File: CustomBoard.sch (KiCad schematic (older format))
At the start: 36 parts, among them J1 RIGHT, J10 Sensor08, J11 Sensor09, J12 Sensor10, J13 Sensor11, J14 Sensor12, J15 Camera, J2 LEFT, J3 Sensor01, J4 Sensor02, J5 Sensor03, J6 Sensor04, J7 Sensor05, J8 Sensor06, J9 Sensor07, U1 DS28E05, U2 PCA9555, U3 VL53L1X

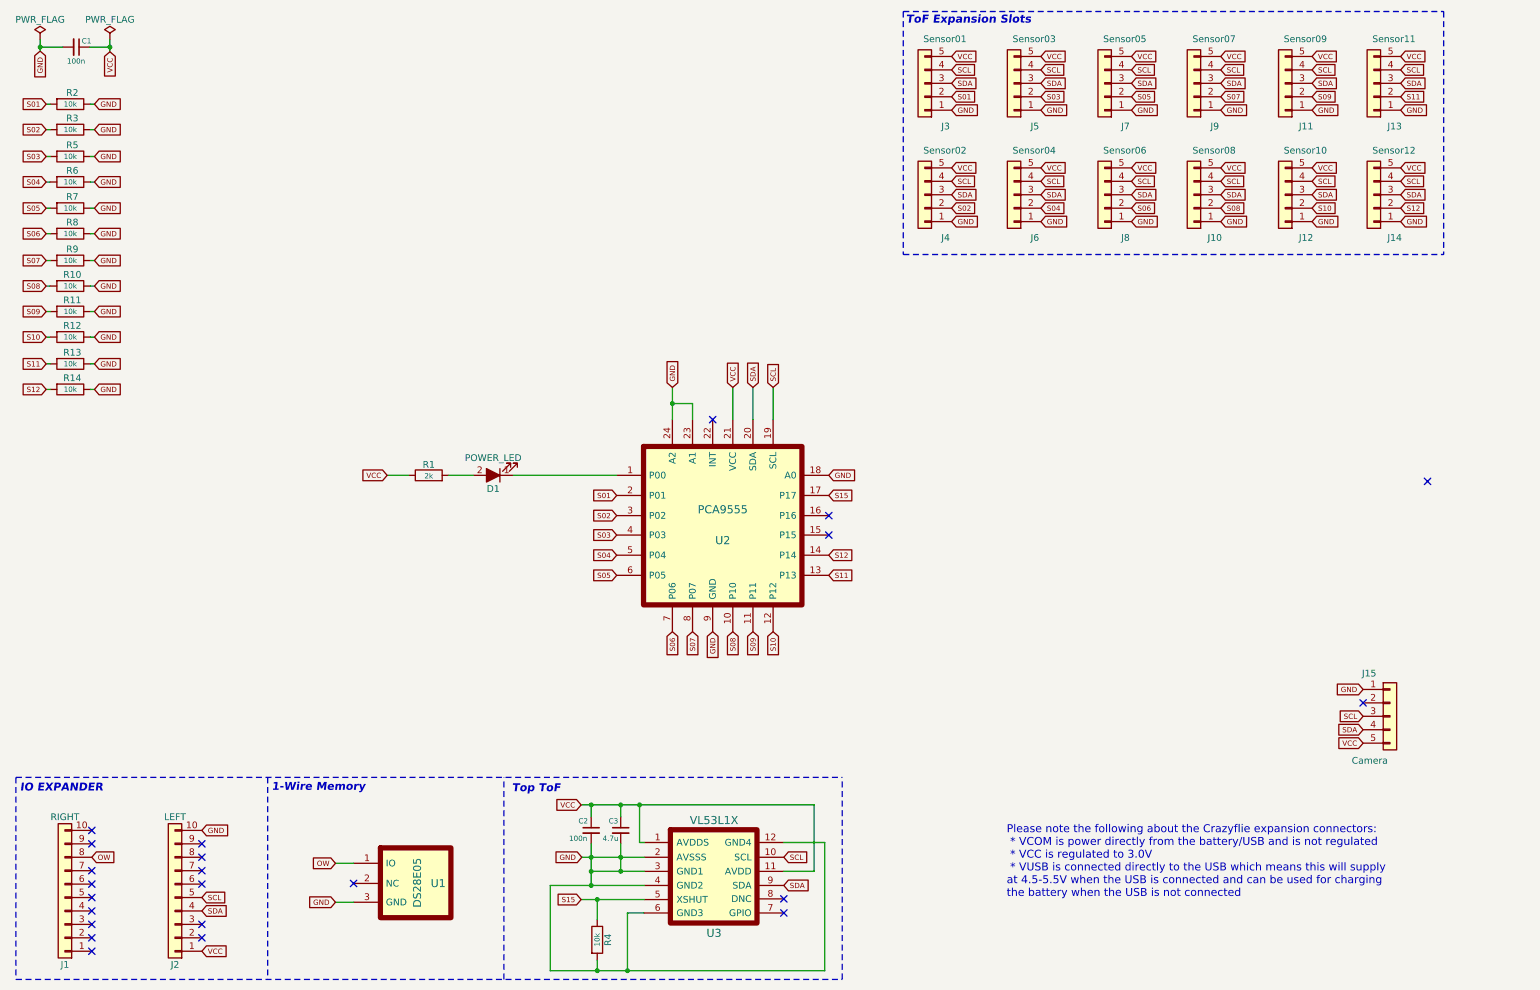
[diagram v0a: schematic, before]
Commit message: reformatting
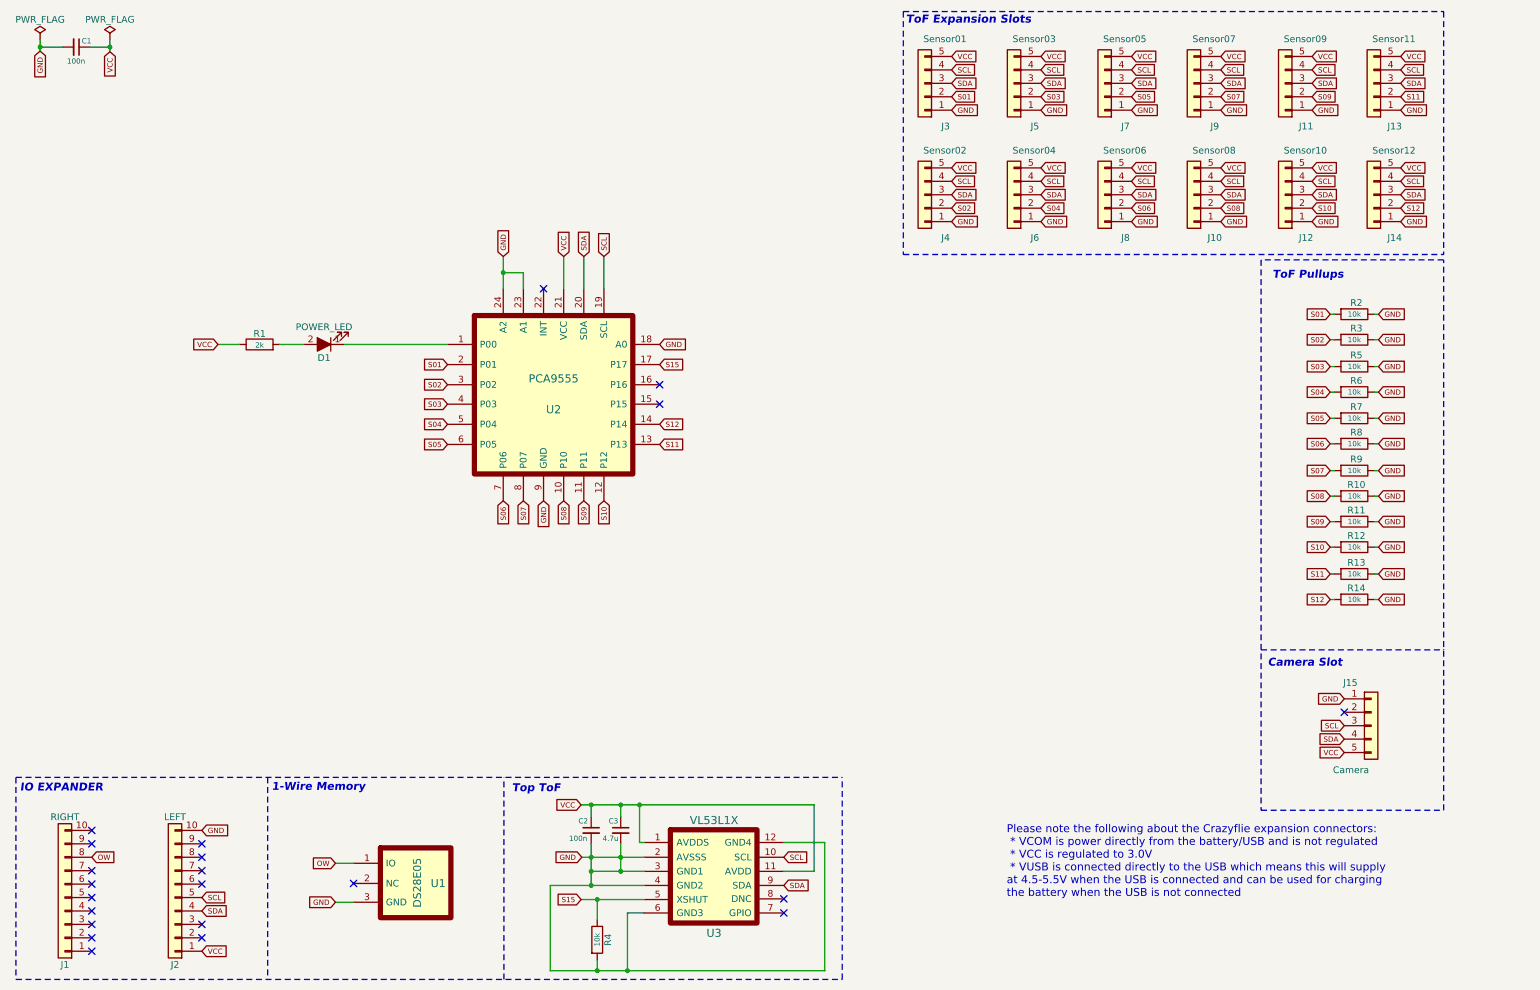
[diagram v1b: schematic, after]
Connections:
- no-connect marks 23 -> 22
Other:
- note added: "Camera Slot"
- note added: "ToF Pullups"
- moved on the sheet: D1, J15, R1, R10, R11, R12, R13, R14, R2, R3, R5, R6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
